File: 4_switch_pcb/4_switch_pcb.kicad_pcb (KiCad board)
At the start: 2 copper layers, 27 parts, among them J1 USB_B_Micro, J2 AVR-ISP-6, J3 Conn_01x03_Pin, SW1 SW_Push, SW2 SW_Push, SW3 SW_Push, SW4 SW_Push, SW5 SW_Push, U1 ATmega32U4-A, Y1 Crystal 16Mhz

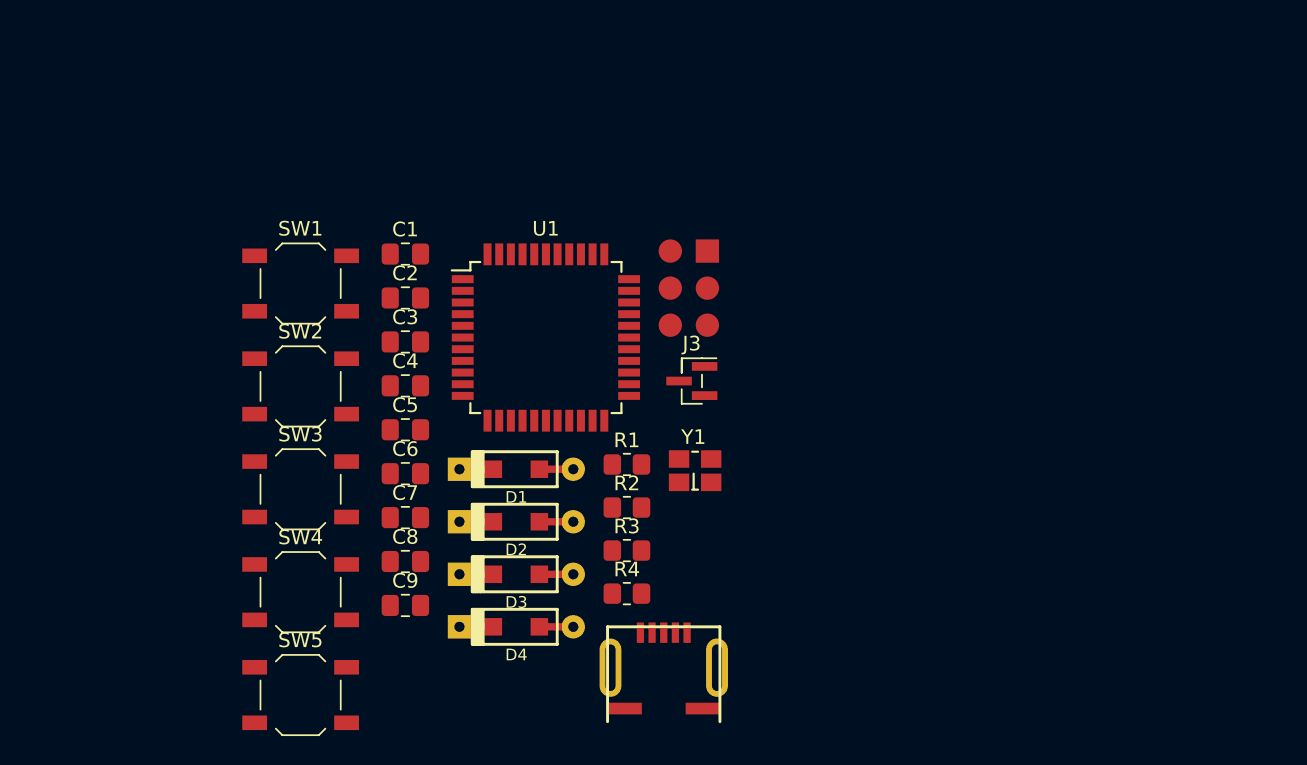
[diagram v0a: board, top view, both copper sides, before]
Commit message: component alignement
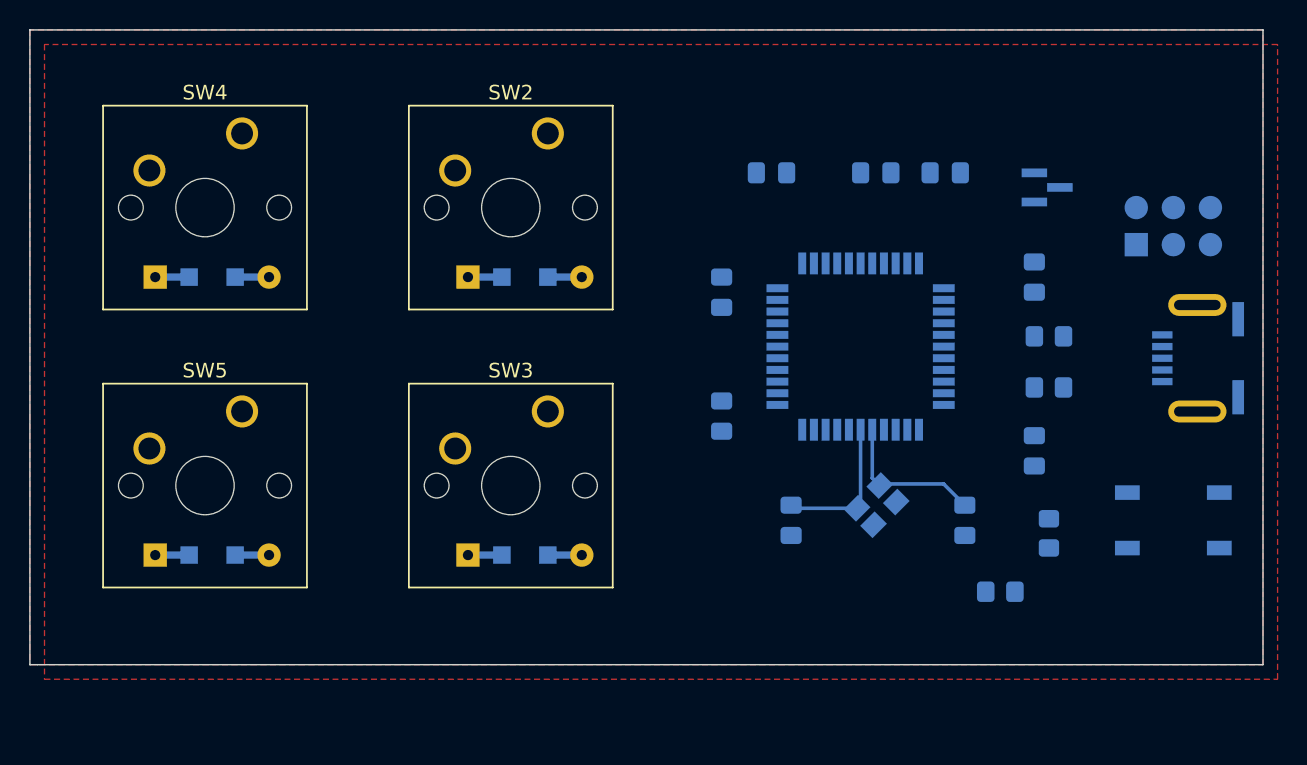
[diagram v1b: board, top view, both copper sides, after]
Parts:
- C1, C2, C3, C4, C5, C6, C7, C8, C9, D1, D2, D3, D4, J1, J2, J3, R1, R2, R3, R4, SW1, U1, Y1: moved to B.Cu
- SW2, SW3, SW4, SW5: footprint Button_Switch_SMD:SW_SPST_TL3342 -> Button_Switch_Keyboard:SW_Cherry_MX_1.00u_PCB
- moved SW1 62.0 mm to (183.4, 88.1), turned to 180 degrees
- moved C8 47.3 mm to (173.8, 71.4), turned to -90 degrees
- moved C4 43.3 mm to (173.8, 83.3), turned to -90 degrees
- moved C1 42.5 mm to (169.1, 88.1), turned to -90 degrees
- moved C6 42.4 mm to (167.7, 64.3), turned to 180 degrees
- moved J1 39.0 mm to (182.6, 77.0), turned to -90 degrees
- moved C3 34.3 mm to (163.0, 64.3), turned to 180 degrees
- moved R3 32.4 mm to (174.8, 75.5), turned to 180 degrees
- moved R4 32.2 mm to (174.8, 79.0), turned to 180 degrees
- moved J2 32.1 mm to (180.8, 66.7), turned to -90 degrees
- moved SW4 31.7 mm to (119.5, 61.6)
- moved C5 30.7 mm to (155.8, 64.3), turned to 180 degrees
- moved C2 30.5 mm to (157.2, 88.1), turned to -90 degrees
- moved C9 30.5 mm to (152.4, 72.5), turned to -90 degrees
- moved R2 29.0 mm to (174.8, 89.0), turned to -90 degrees
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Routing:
- net Net-(U1-XTAL2): track 0.00 -> 10.5 mm
- net Net-(U1-XTAL1): track 0.00 -> 10.1 mm
- added copper zone on F.Cu, net GND
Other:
- board outline added: 84.5 x 43.5 mm

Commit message: add base of routing
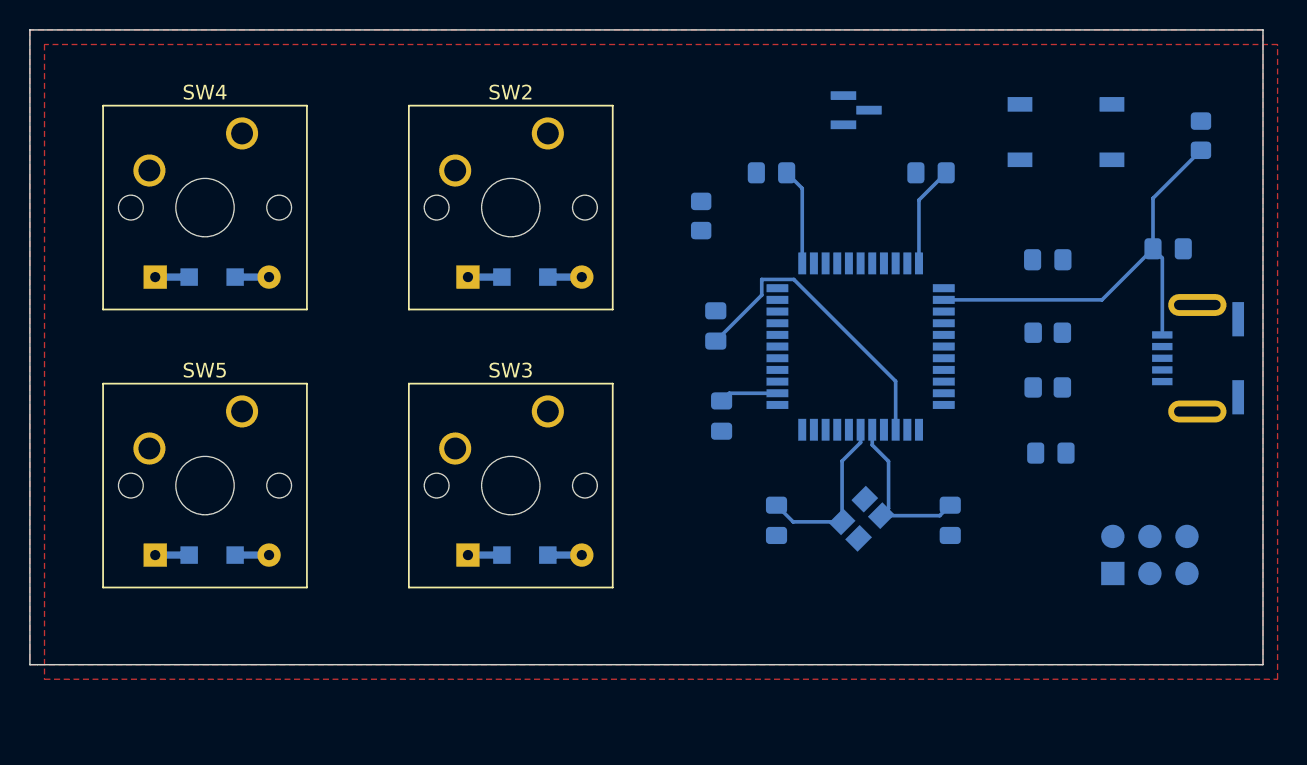
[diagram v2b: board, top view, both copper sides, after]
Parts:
- removed Y1: Crystal 16Mhz, user:crystal_FA238-TSX3225
- added X1: 16 MHZ, user:crystal_FA238-TSX3225, B.Cu at (162.0, 88.0)
- C8: value 100nF -> 4.7uF
- moved R1 34.1 mm to (185.2, 61.8), turned to 90 degrees
- moved R2 32.3 mm to (151.0, 67.2), turned to 90 degrees
- moved SW1 27.6 mm to (176.0, 61.5)
- moved C4 23.4 mm to (152.0, 74.8), turned to 90 degrees
- moved C3 22.6 mm to (175.0, 83.5)
- moved J2 22.6 mm to (179.2, 89.2)
- moved C9 22.5 mm to (174.8, 70.2), turned to 180 degrees
- moved J3 14.1 mm to (161.6, 60.0)
- moved C8 9.37 mm to (183.0, 69.5), turned to 0 degrees
- moved R4 3.75 mm to (174.8, 75.2)
- moved R3 3.50 mm to (174.8, 79.0)
- moved C1 1.00 mm to (168.1, 88.1)
- moved C2 1.00 mm to (156.2, 88.1)
- moved C6 0.97 mm to (166.8, 64.3)
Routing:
- net VCC: track 0.00 -> 68.7 mm
- net Net-(U1-XTAL1): track 10.1 -> 11.8 mm
- net Net-(U1-XTAL2): track 10.5 -> 11.6 mm
